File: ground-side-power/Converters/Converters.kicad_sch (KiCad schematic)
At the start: 41 parts, among them J10 Conn_01x03_Female, J11 Ground Connections, J12 Conn_01x04_Female, J13 DAQ Voltage Sensing, J14 DAQ Current Sensing, J27 Conn_01x02_Female, U1 TPS55340, U2 K7805-3AR3, U4 INA180, U5 INA180

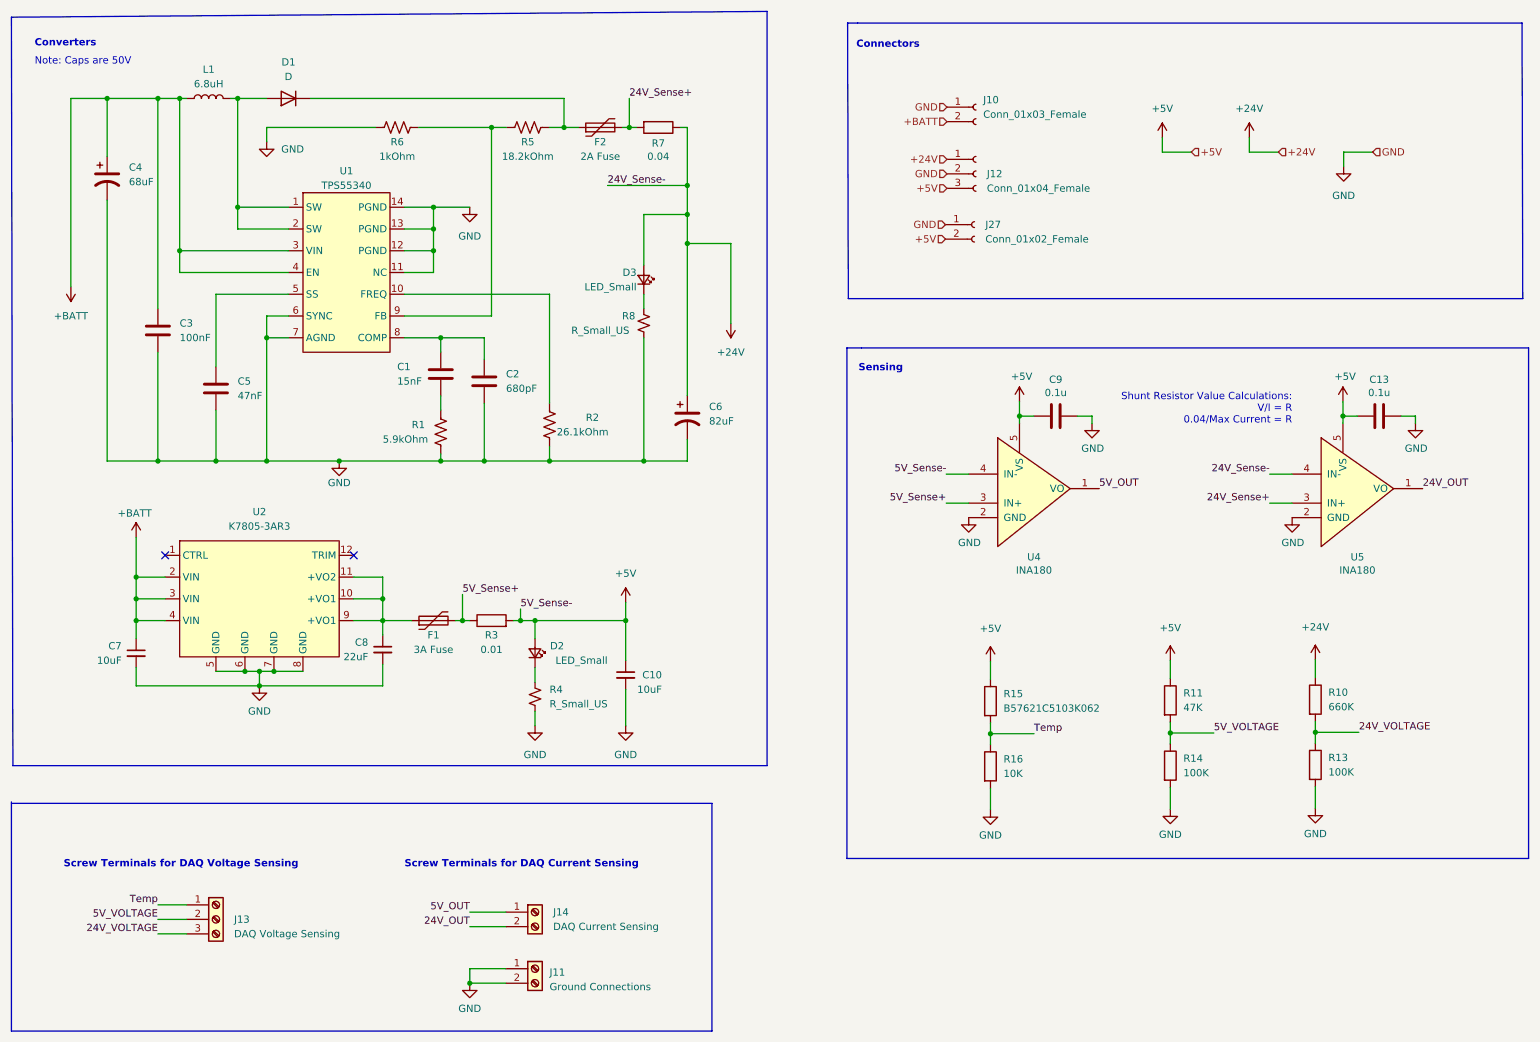
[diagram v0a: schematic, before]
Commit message: implemented comments
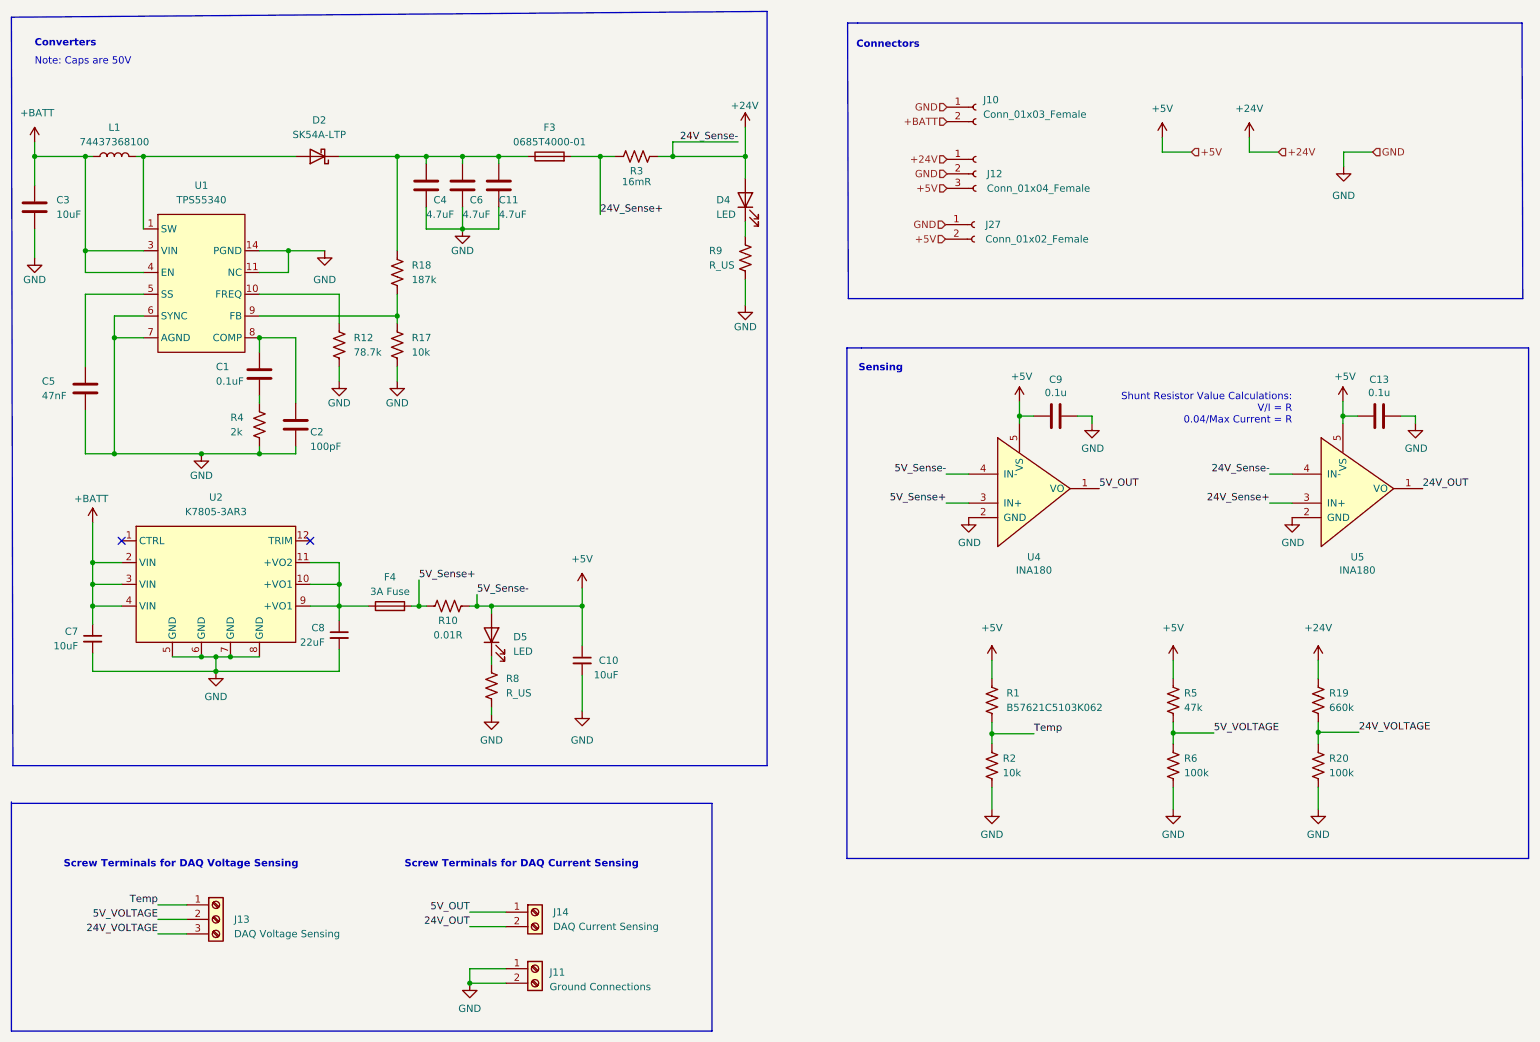
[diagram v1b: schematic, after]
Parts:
- removed C4: 68uF, Capacitor_SMD:C_Elec_6.3x7.7, symbol Device:C_Polarized_US
- removed C6: 82uF, Capacitor_SMD:CP_Elec_8x11.9, symbol Device:C_Polarized_US
- removed D1: D, Diode_SMD:D_SMB-SMC_Universal_Handsoldering, symbol Device:D
- removed D2, D3: LED_Small, Diode_SMD:D_1206_3216Metric_Pad1.42x1.75mm_HandSolder, symbol Device:LED_Small
- removed F1: 3A Fuse, Fuse:Fuseholder_Clip-6.3x32mm_Littelfuse_102_122_Inline_P34.21x7.62mm_D1.98mm_Horizontal, symbol Device:Polyfuse
- removed F2: 2A Fuse, Fuse:Fuseholder_Clip-6.3x32mm_Littelfuse_102_122_Inline_P34.21x7.62mm_D1.98mm_Horizontal, symbol Device:Polyfuse
- removed R10: 660K, Resistor_SMD:R_0805_2012Metric_Pad1.20x1.40mm_HandSolder, symbol Device:R
- removed R11: 47K, Resistor_SMD:R_0805_2012Metric_Pad1.20x1.40mm_HandSolder, symbol Device:R
- removed R13, R14: 100K, Resistor_SMD:R_0805_2012Metric_Pad1.20x1.40mm_HandSolder, symbol Device:R
- removed R15: B57621C5103K062, Resistor_SMD:R_1206_3216Metric_Pad1.30x1.75mm_HandSolder, symbol Device:R
- removed R16: 10K, Resistor_SMD:R_0805_2012Metric_Pad1.20x1.40mm_HandSolder, symbol Device:R
- removed R3: 0.01, Resistor_SMD:R_2512_6332Metric_Pad1.40x3.35mm_HandSolder, symbol Device:R
- removed R4, R8: R_Small_US, Resistor_SMD:R_0805_2012Metric_Pad1.20x1.40mm_HandSolder, symbol Device:R_Small_US
- removed R7: 0.04, Resistor_SMD:R_2512_6332Metric_Pad1.40x3.35mm_HandSolder, symbol Device:R
- added C11, C4, C6: 4.7uF, Capacitor_SMD:C_0805_2012Metric_Pad1.18x1.45mm_HandSolder, symbol Device:C
- added D2: SK54A-LTP, symbol Device:D_Schottky
- added D4, D5: LED, symbol Device:LED
- added F3: 0685T4000-01, symbol Device:Fuse
- added F4: 3A Fuse, symbol Device:Fuse
- added R10: 0.01R, symbol Device:R_US
- added R12: 78.7k, symbol Device:R_US
- added R17: 10k, symbol Device:R_US
- added R18: 187k, symbol Device:R_US
- added R19: 660k, symbol Device:R_US
- added R20: 100k, symbol Device:R_US
- added R3: 16mR, symbol Device:R_US
- added R4: 2k, symbol Device:R_US
- added R8, R9: R_US, symbol Device:R_US
- C1: value 15nF -> 0.1uF
- C2: value 680pF -> 100pF
- C3: value 100nF -> 10uF
- L1: value 6.8uH -> 74437368100
- R1: value 5.9kOhm -> B57621C5103K062; footprint Resistor_SMD:R_0402_1005Metric_Pad0.72x0.64mm_HandSolder -> (none)
- R2: value 26.1kOhm -> 10k; footprint Resistor_SMD:R_0402_1005Metric_Pad0.72x0.64mm_HandSolder -> (none)
- R5: value 18.2kOhm -> 47k; footprint Resistor_SMD:R_0402_1005Metric_Pad0.72x0.64mm_HandSolder -> (none)
- R6: value 1kOhm -> 100k; footprint Resistor_SMD:R_0402_1005Metric_Pad0.72x0.64mm_HandSolder -> (none)
- U1: footprint Package_SO:TSSOP-14_4.4x3.6mm_P0.4mm -> (none)
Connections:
- net +24V: now also D4.2 (A), R19.1, R3.2
- net +5V: now also R1.1, R5.1, D5.2 (A), R10.2
- net 24V_Sense+: now also F3.2, R3.1
- net 24V_VOLTAGE: now also R19.2, R20.1
- net 5V_Sense+: now also F4.2, R10.1
- net 5V_VOLTAGE: now also R5.2, R6.1
- net GND: now also R6.2, C11.2, C4.2, C6.2, R12.2, R17.2, R20.2, R4.2, R8.2, R9.2; no longer R1.2, R6.1
- net Temp: now also R1.2, R2.1
- net at C1.2: now also R4.1; no longer R1.1
- net at C8.1, U2.10 (+VO1), U2.11 (+VO2)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: now also F4.1
- net at L1.2, U1.1 (SW), U1.2 (SW): now also D2.2 (A)
- net at U1.10 (FREQ): now also R12.1; no longer R2.1
- new net: R17.1, R18.1, U1.9 (FB)
- new net: C11.1, C4.1, C6.1, D2.1 (K), F3.1, R18.2
- new net: D4.1 (K), R9.1
- new net: D5.1 (K), R8.1
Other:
- moved on the sheet: C1, C10, C2, C3, C5, C7, C8, L1, U2
